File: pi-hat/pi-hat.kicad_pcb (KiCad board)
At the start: 2 copper layers, 65 x 56 mm, 18 parts, among them J10 Conn_01x02_Pin, J11 Conn_01x02_Pin, J12 Conn_01x02_Pin, J3 Conn_01x02_Pin, J4 Conn_01x02_Pin, J5 Conn_01x02_Pin, J6 Conn_01x02_Pin, J7 Conn_01x02_Pin, J8 GPIO, SW1 SW_Push

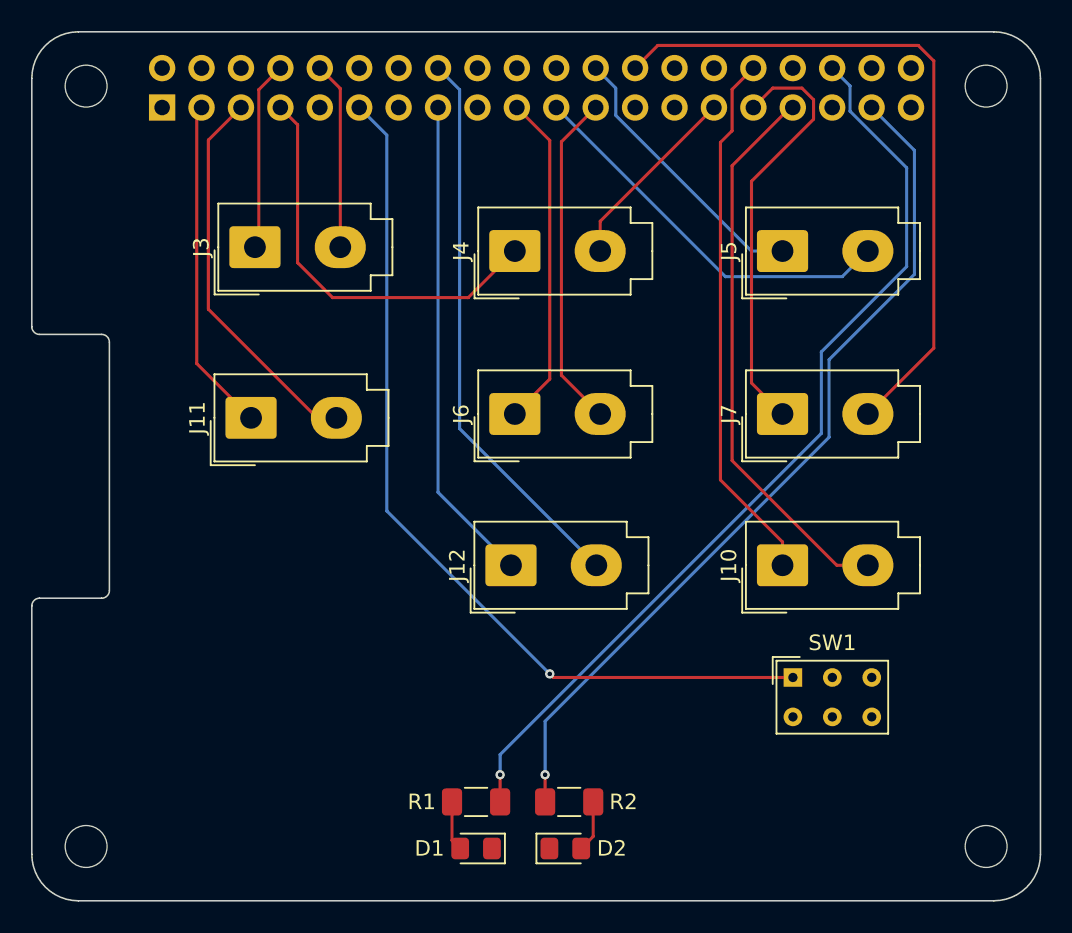
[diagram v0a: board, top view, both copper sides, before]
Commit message: Update Layout Rules, and Cleanup a bit
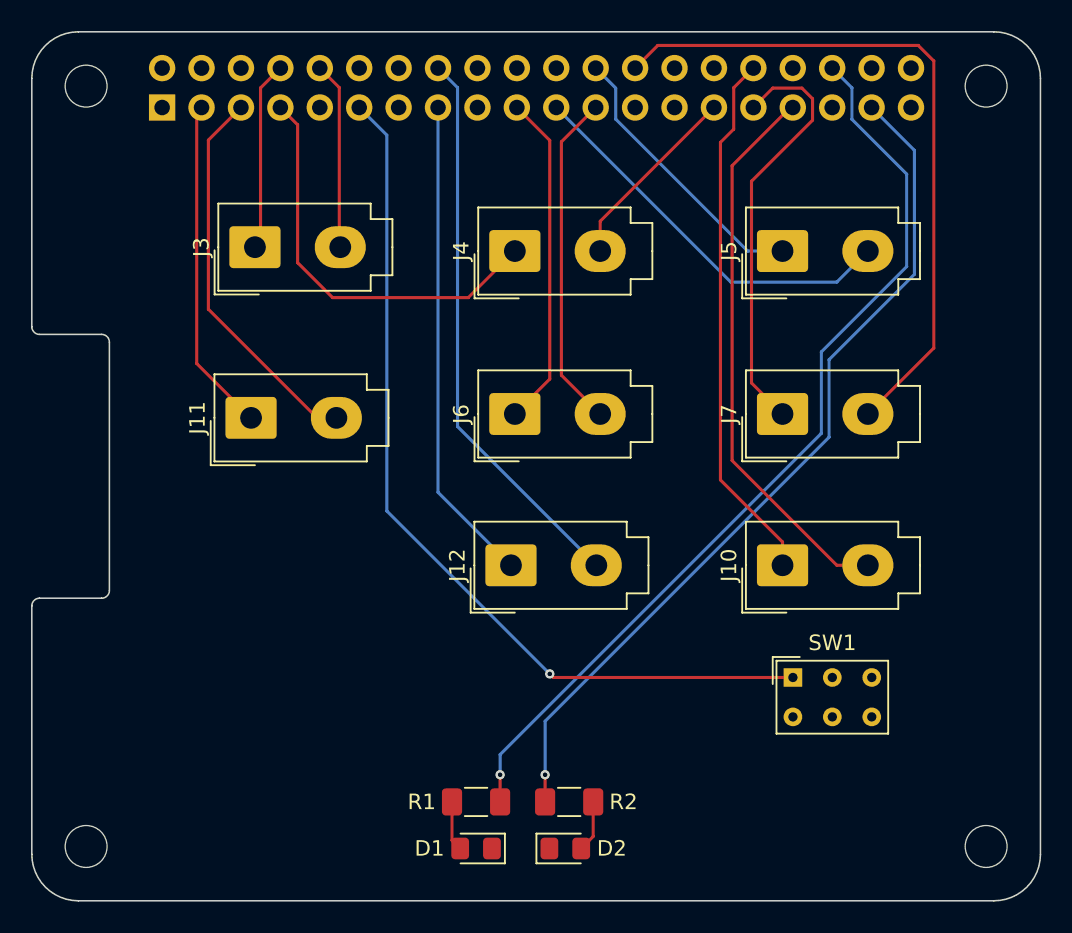
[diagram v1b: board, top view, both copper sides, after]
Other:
- rule pad_to_mask_clearance: 0 -> 0.09
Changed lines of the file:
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@@
 	)
 	(setup
-		(pad_to_mask_clearance 0)
+		(stackup
+			(layer "F.SilkS"
+				(type "Top Silk Screen")
+			)
+			(layer "F.Paste"
+				(type "Top Solder Paste")
+			)
+			(layer "F.Mask"
+				(type "Top Solder Mask")
+				(thickness 0.01)
+			)
+			(layer "F.Cu"
+				(type "copper")
+				(thickness 0.035)
+			)
+			(layer "dielectric 1"
+				(type "core")
+				(thickness 1.51)
+				(material "FR4")
+				(epsilon_r 4.5)
+				(loss_tangent 0.02)
+			)
+			(layer "B.Cu"
+				(type "copper")
+				(thickness 0.035)
+			)
+			(layer "B.Mask"
+				(type "Bottom Solder Mask")
+				(thickness 0.01)
+			)
+			(layer "B.Paste"
+				(type "Bottom Solder Paste")
+			)
+			(layer "B.SilkS"
+				(type "Bottom Silk Screen")
+			)
+			(copper_finish "None")
+			(dielectric_constraints no)
+		)
+		(pad_to_mask_clearance 0.09)
 		(allow_soldermask_bridges_in_footprints no)
 		(tenting
@@
 		(capping no)
 		(filling no)
+		(zone_defaults)
 		(pcbplotparams
 			(layerselection 0x00000000_00000000_55555555_5755f5ff)
@@
 	)
 	(segment
-		(start 88 51.5)
-		(end 88.25 51.25)
+		(start 88.360671 41.239329)
+		(end 89.64 39.96)
 		(width 0.2)
 		(layer "F.Cu")
@@
 	)
 	(segment
-		(start 88.25 51.25)
-		(end 88.25 41.35)
+		(start 88.360671 51.139329)
+		(end 88.360671 41.239329)
 		(width 0.2)
 		(layer "F.Cu")
@@
 	)
 	(segment
-		(start 88.25 41.35)
-		(end 89.64 39.96)
+		(start 88 51.5)
+		(end 88.360671 51.139329)
 		(width 0.2)
 		(layer "F.Cu")
@@
 	)
 	(segment
+		(start 93.437707 51.437707)
+		(end 93.437707 41.217707)
+		(width 0.2)
+		(layer "F.Cu")
+		(net "/PI-HAT/GPIO15{slash}RXD0")
+	)
+	(segment
 		(start 93.5 51.5)
-		(end 93.5 41.28)
+		(end 93.437707 51.437707)
 		(width 0.2)
 		(layer "F.Cu")
@@
 	)
 	(segment
-		(start 93.5 41.28)
+		(start 93.437707 41.217707)
 		(end 92.18 39.96)
 		(width 0.2)
@@
 	)
 	(segment
-		(start 122 51.75)
-		(end 120 51.75)
+		(start 119.75 51.75)
+		(end 111.25 43.25)
 		(width 0.2)
 		(layer "B.Cu")
@@
 	)
 	(segment
-		(start 111.25 43)
-		(end 111.25 41.25)
+		(start 122 51.75)
+		(end 119.75 51.75)
 		(width 0.2)
 		(layer "B.Cu")
@@
 	)
 	(segment
-		(start 120 51.75)
-		(end 111.25 43)
+		(start 111.25 43.25)
+		(end 111.25 41.25)
 		(width 0.2)
 		(layer "B.Cu")
@@
 	(segment
 		(start 127.5 51.75)
-		(end 125.85 53.4)
+		(end 125.5 53.75)
 		(width 0.2)
 		(layer "B.Cu")
@@
 	)
 	(segment
-		(start 118.32 53.4)
+		(start 118.67 53.75)
 		(end 107.42 42.5)
 		(width 0.2)
@@
 	)
 	(segment
-		(start 125.85 53.4)
-		(end 118.32 53.4)
+		(start 125.5 53.75)
+		(end 118.67 53.75)
 		(width 0.2)
 		(layer "B.Cu")
@@
 	)
 	(segment
-		(start 123.25 41.25)
-		(end 121.37 41.25)
+		(start 122 62.25)
+		(end 120 60.25)
 		(width 0.2)
 		(layer "F.Cu")
@@
 	)
 	(segment
-		(start 124 43.25)
-		(end 124 42)
+		(start 123.93367 43.31633)
+		(end 123.93367 41.93367)
 		(width 0.2)
 		(layer "F.Cu")
@@
 	)
 	(segment
-		(start 124 42)
+		(start 123.93367 41.93367)
 		(end 123.25 41.25)
 		(width 0.2)
@@
 	)
 	(segment
-		(start 122 62.25)
-		(end 120 60.25)
+		(start 120 60.25)
+		(end 120 47.25)
 		(width 0.2)
 		(layer "F.Cu")
@@
 	)
 	(segment
-		(start 120 47.25)
-		(end 124 43.25)
+		(start 123.25 41.25)
+		(end 121.37 41.25)
 		(width 0.2)
 		(layer "F.Cu")
@@
 	)
 	(segment
-		(start 120 60.25)
-		(end 120 47.25)
+		(start 120 47.25)
+		(end 123.93367 43.31633)
 		(width 0.2)
 		(layer "F.Cu")
@@
 	)
 	(segment
-		(start 122 72)
-		(end 122 70.5)
+		(start 118.85364 41.22636)
+		(end 120.12 39.96)
 		(width 0.2)
 		(layer "F.Cu")
@@
 	)
 	(segment
-		(start 118.75 44)
-		(end 118.75 41.33)
+		(start 122 70.5)
+		(end 118 66.5)
 		(width 0.2)
 		(layer "F.Cu")
@@
 	(segment
 		(start 118 44.75)
-		(end 118.75 44)
+		(end 118.85364 43.89636)
 		(width 0.2)
 		(layer "F.Cu")
@@
 	)
 	(segment
-		(start 122 70.5)
-		(end 118 66.5)
+		(start 122 72)
+		(end 122 70.5)
 		(width 0.2)
 		(layer "F.Cu")
@@
 	)
 	(segment
-		(start 118.75 41.33)
-		(end 120.12 39.96)
+		(start 118.85364 43.89636)
+		(end 118.85364 41.22636)
 		(width 0.2)
 		(layer "F.Cu")
@@
 	)
 	(segment
-		(start 101.19 41.35)
-		(end 99.8 39.96)
+		(start 101.056165 63.056165)
+		(end 101.056165 41.216165)
 		(width 0.2)
 		(layer "B.Cu")
@@
 	)
 	(segment
-		(start 101.19 63.19)
-		(end 101.19 41.35)
+		(start 110 72)
+		(end 101.056165 63.056165)
 		(width 0.2)
 		(layer "B.Cu")
@@
 	)
 	(segment
-		(start 110 72)
-		(end 101.19 63.19)
+		(start 101.056165 41.216165)
+		(end 99.8 39.96)
 		(width 0.2)
 		(layer "B.Cu")
@@
 	)
 	(segment
-		(start 130 52.75)
-		(end 130 46.386346)
+		(start 103.8 84.2)
+		(end 124.5 63.5)
 		(width 0.2)
 		(layer "B.Cu")
@@
 	)
 	(segment
-		(start 124.5 58.25)
-		(end 130 52.75)
+		(start 124.5 63.5)
+		(end 124.5 58.25)
 		(width 0.2)
 		(layer "B.Cu")
@@
 	)
 	(segment
-		(start 130 46.386346)
-		(end 126.35 42.736346)
+		(start 130 52.75)
+		(end 130 46.790555)
 		(width 0.2)
 		(layer "B.Cu")
@@
 	)
 	(segment
-		(start 103.8 84.2)
-		(end 124.5 63.5)
+		(start 126.471521 43.262076)
+		(end 126.471521 41.231521)
 		(width 0.2)
 		(layer "B.Cu")
@@
 	)
 	(segment
-		(start 126.35 41.11)
+		(start 126.471521 41.231521)
 		(end 125.2 39.96)
 		(width 0.2)
@@
 	)
 	(segment
-		(start 124.5 63.5)
-		(end 124.5 58.25)
+		(start 124.5 58.25)
+		(end 130 52.75)
 		(width 0.2)
 		(layer "B.Cu")
@@
 	)
 	(segment
-		(start 126.35 42.736346)
-		(end 126.35 41.11)
+		(start 130 46.790555)
+		(end 126.471521 43.262076)
 		(width 0.2)
 		(layer "B.Cu")
